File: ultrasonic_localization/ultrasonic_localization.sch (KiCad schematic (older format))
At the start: 22 parts

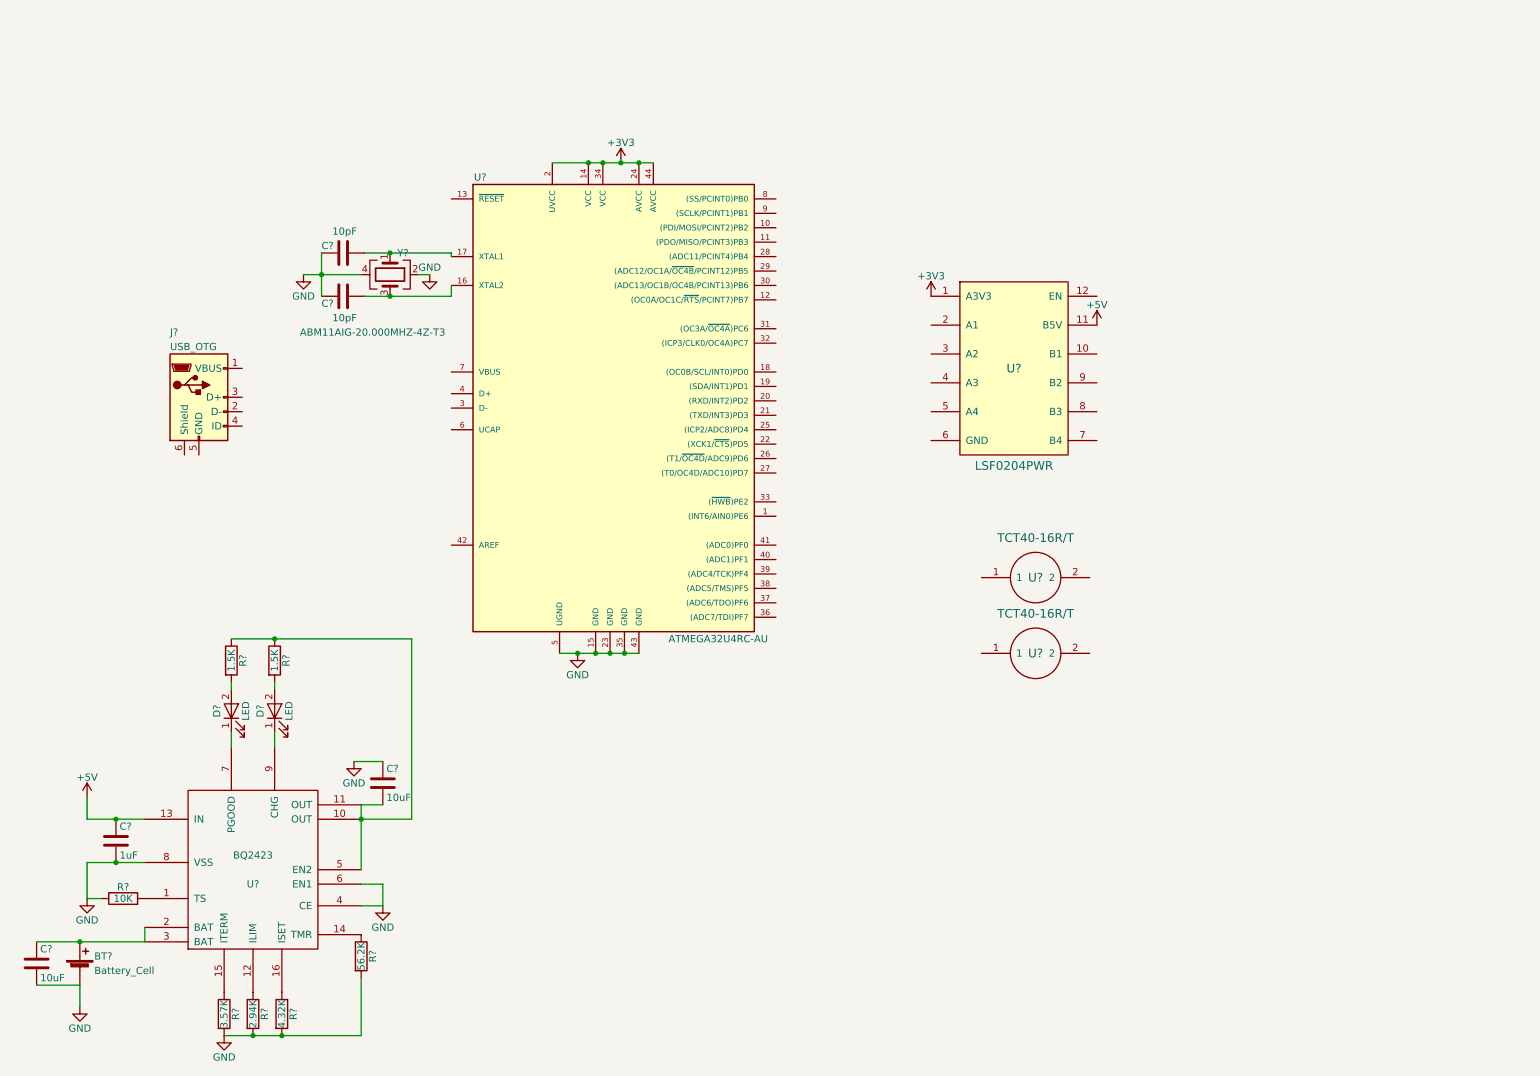
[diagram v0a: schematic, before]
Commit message: adding more cxns
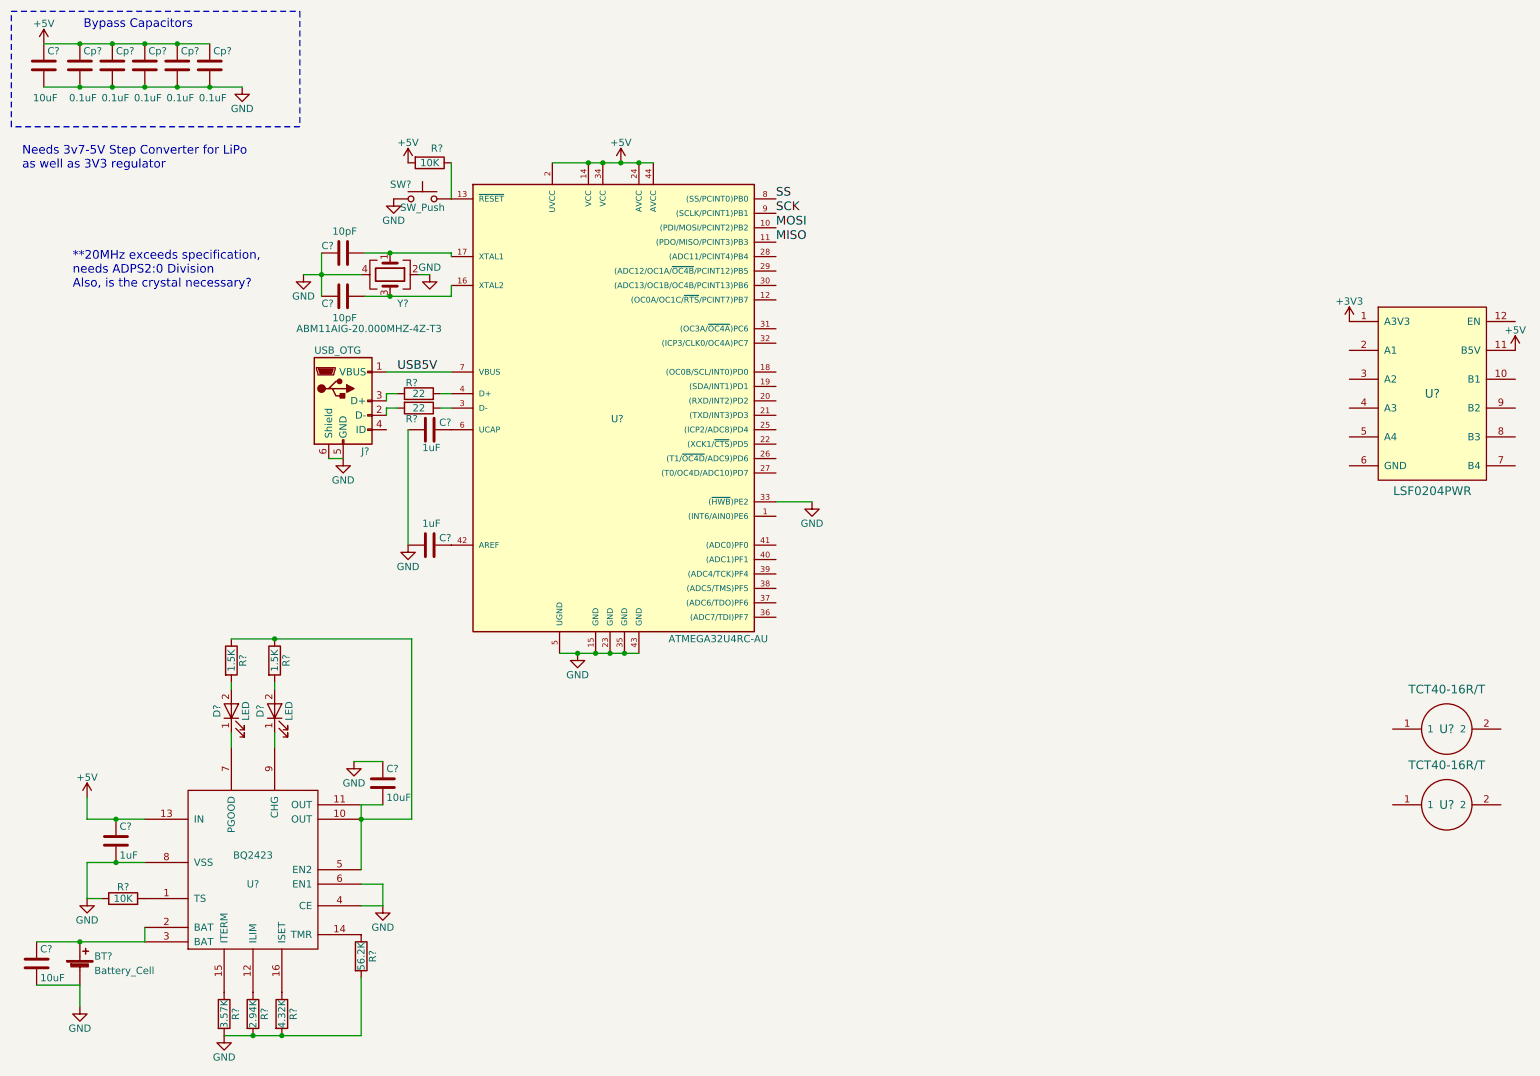
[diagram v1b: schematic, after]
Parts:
- added C? (x2): 1uF, symbol C
- added C?: 10uF, symbol C
- added Cp? (x5): 0.1uF, symbol C
- added R?: 10K, symbol R
- added R? (x2): 22, symbol R
- added SW?: SW_Push, symbol SW_Push
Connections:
- net +3V3: no longer U?.14 (VCC), U?.2 (UVCC), U?.24 (AVCC), U?.34 (VCC), U?.44 (AVCC)
- net +5V: now also U?.14 (VCC), U?.2 (UVCC), U?.24 (AVCC), U?.34 (VCC), U?.44 (AVCC), C?.1, Cp?.1, Cp?.1, Cp?.1, Cp?.1, Cp?.1, R?.2
- net GND: now also J?.5 (GND), J?.6 (Shield), U?.33 ((~HWB~)PE2), C?.1, C?.1, C?.2, Cp?.2, Cp?.2, Cp?.2, Cp?.2, Cp?.2, SW?.1
- net MOSI: now reaches U?.10 ((PDI/MOSI/PCINT2)PB2)
- net MISO: now reaches U?.11 ((PDO/MISO/PCINT3)PB3)
- net at U?.13 (~RESET~): now also R?.1, SW?.2
- net at U?.3 (D-): now also R?.1
- net at U?.4 (D+): now also R?.2
- net at U?.42 (AREF): now also C?.2
- net at U?.6 (UCAP): now also C?.2
- net USB5V: now reaches U?.7 (VBUS)
- net USB5V: now also J?.1 (VBUS)
- net SS: now reaches U?.8 ((SS/PCINT0)PB0)
- net SCK: now reaches U?.9 ((SCLK/PCINT1)PB1)
- net at J?.2 (D-): now also R?.2
- net at J?.3 (D+): now also R?.1
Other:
- note added: "**20MHz exceeds specification,\nneeds ADPS2:0 Division\nAlso, is the crystal necessary?"
- note added: "Bypass Capacitors"
- note added: "Needs 3v7-5V Step Converter for LiPo\nas well as 3V3 regulator"
- moved on the sheet: J?, U?
